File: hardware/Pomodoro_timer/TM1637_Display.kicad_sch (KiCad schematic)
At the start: 3 parts, among them U4 CC56-12EWA, U5 TM1637

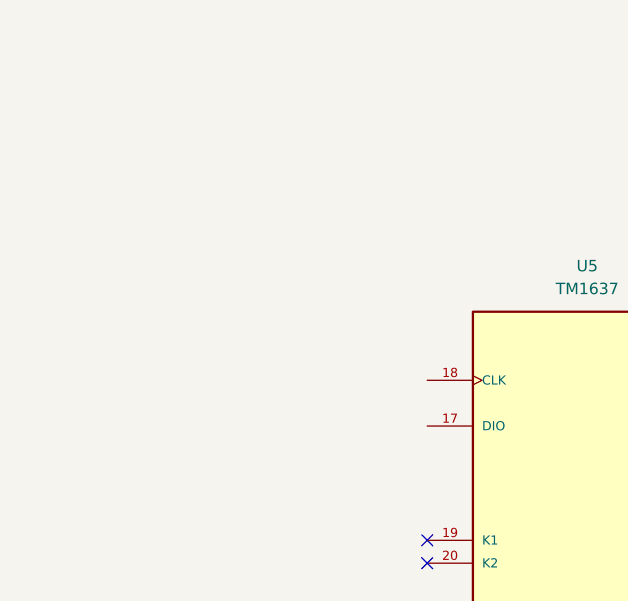
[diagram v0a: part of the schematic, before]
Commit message: PCB Ver.A : The Schematic completed the next part for PCB can be started.
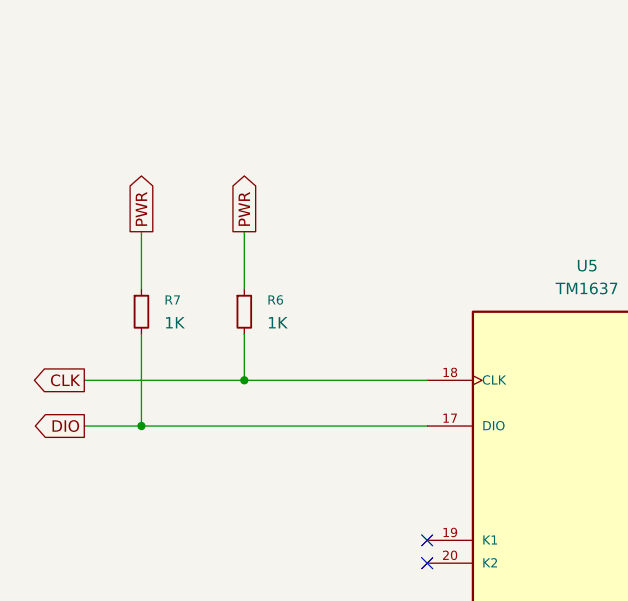
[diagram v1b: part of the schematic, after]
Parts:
- added R6, R7: 1K, symbol Device:R_Small
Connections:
- net PWR: now also R6.1, R7.1
- net DIO: now reaches U5.17 (DIO)
- net DIO: now also R7.2
- net CLK: now reaches U5.18 (CLK)
- net CLK: now also R6.2
